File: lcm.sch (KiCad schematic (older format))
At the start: 13 parts, among them J6 F52R-1A7H1-11020, U11 NTS0102GT

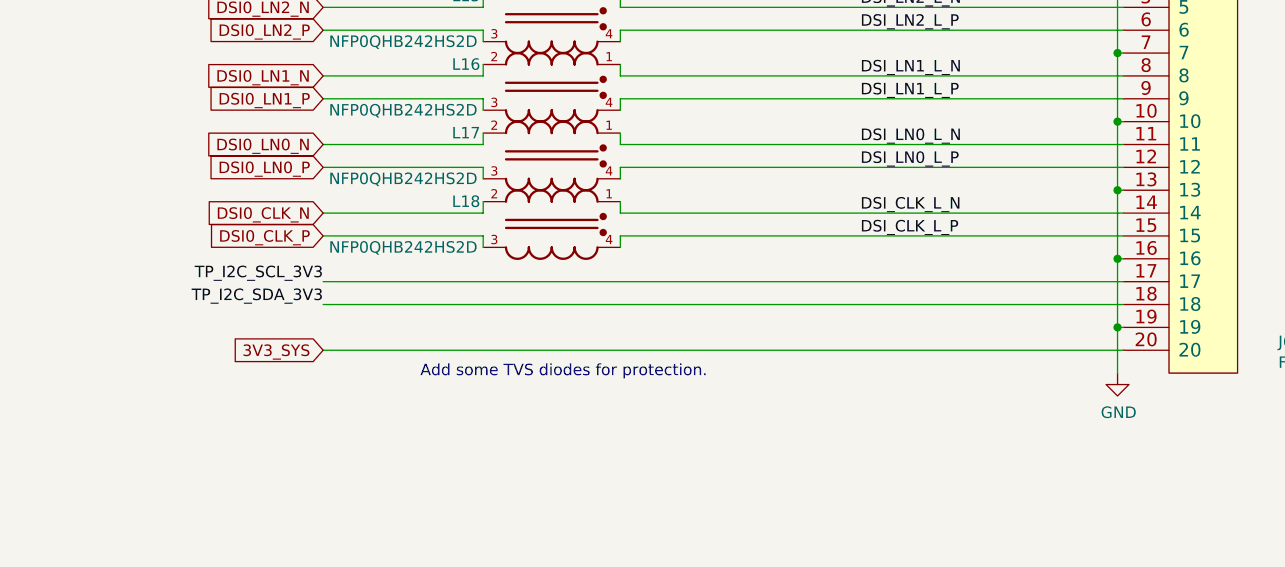
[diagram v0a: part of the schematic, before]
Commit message: Cleanup
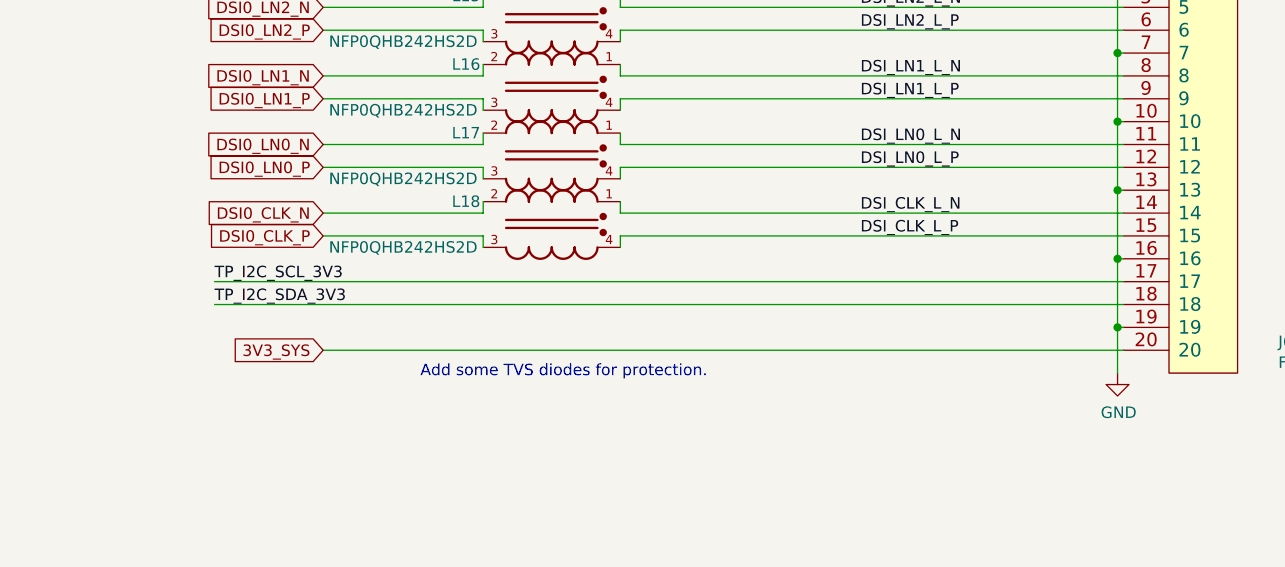
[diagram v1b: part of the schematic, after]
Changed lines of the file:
@@
 $Descr A3 16535 11693
 encoding utf-8
-Sheet 5 13
+Sheet 5 12
 Title ""
 Date ""
@@
 Text Label 5325 7625 2    50   ~ 0
 TP_I2C_SDA_3V3
-Text Label 8025 4600 2    50   ~ 0
+Text Label 7550 4600 0    50   ~ 0
 TP_I2C_SDA_3V3
-Text Label 8025 4500 2    50   ~ 0
+Text Label 7550 4500 0    50   ~ 0
 TP_I2C_SCL_3V3
 $Comp
@@
 	8025 4800 11525 4800
 Wire Wire Line
-	8025 4600 11525 4600
-Wire Wire Line
-	8025 4500 11525 4500
+	7550 4600 11525 4600
+Wire Wire Line
+	7550 4500 11525 4500
 Wire Wire Line
 	9325 4300 11525 4300
